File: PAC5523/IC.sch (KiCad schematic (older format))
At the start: 17 parts

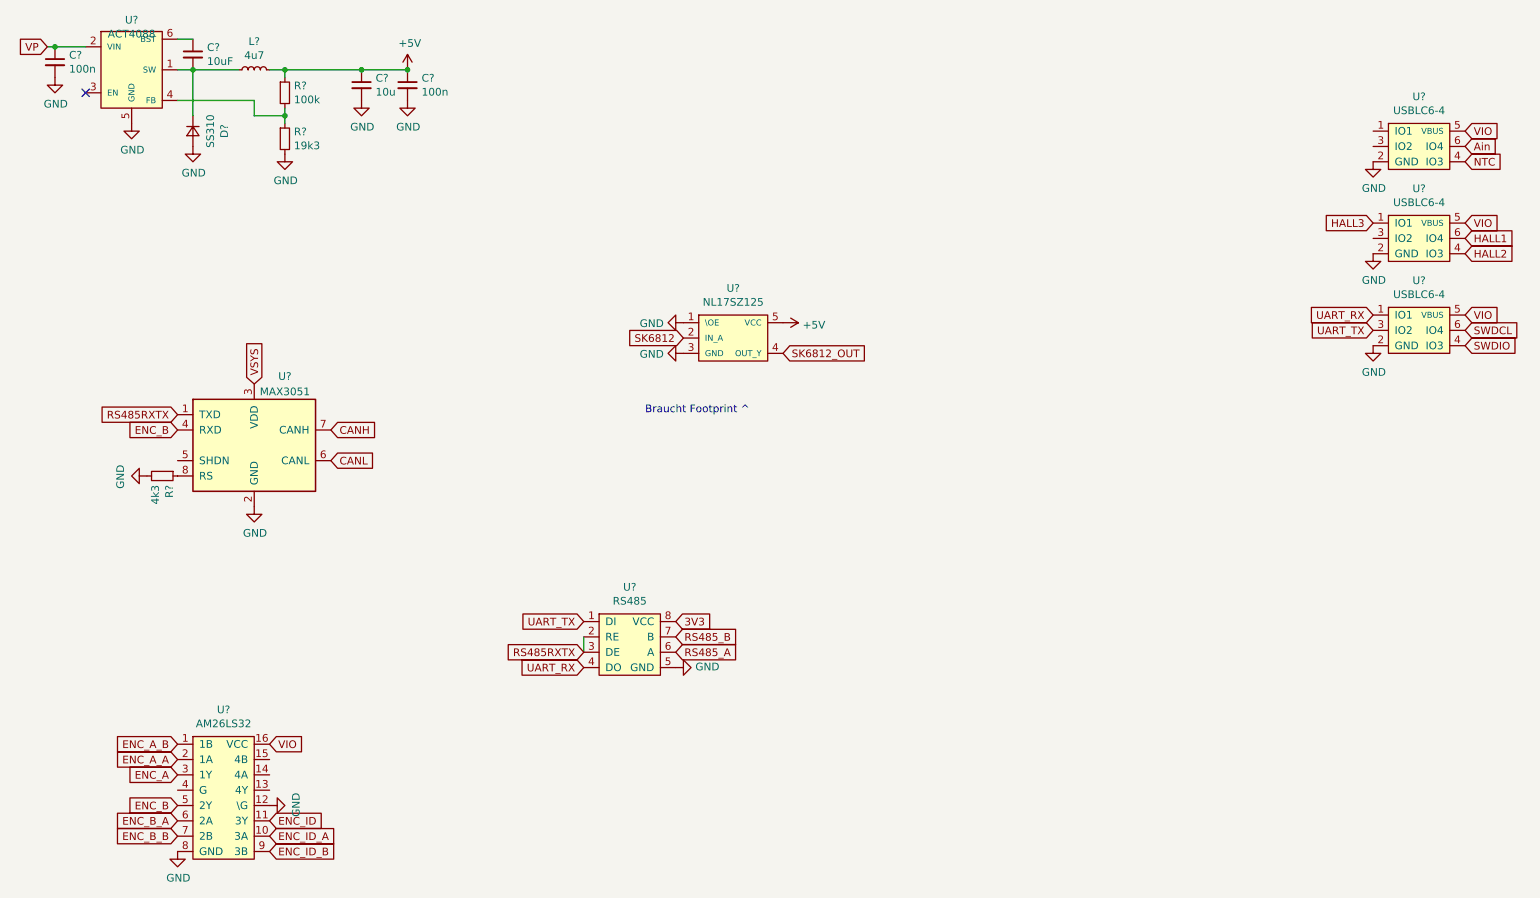
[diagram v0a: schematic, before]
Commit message: updated schematic
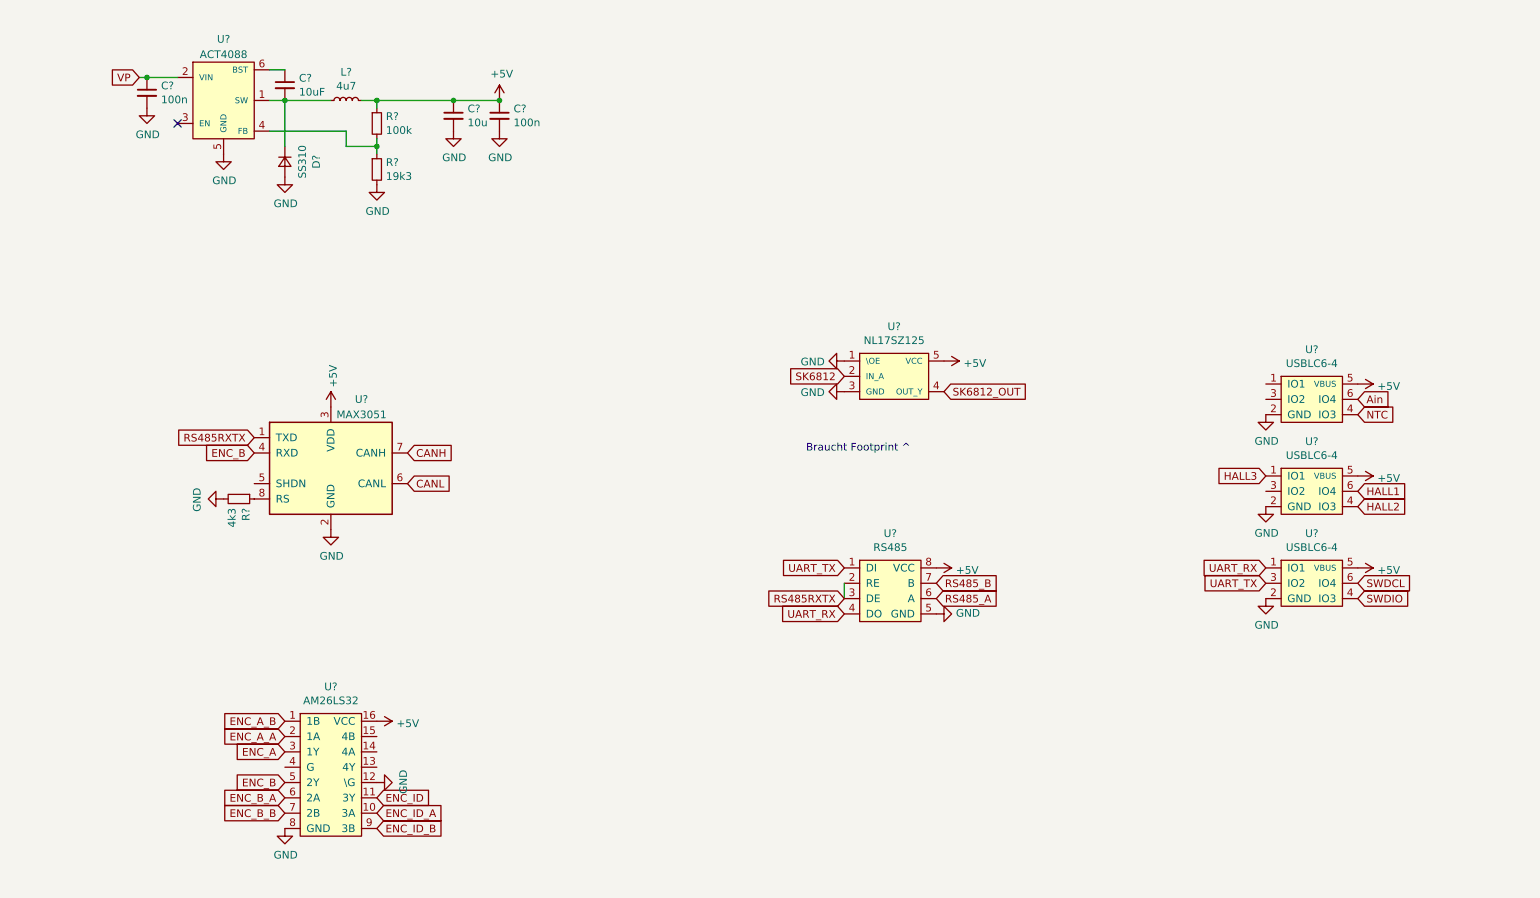
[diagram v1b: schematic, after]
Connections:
- net 3V3 is gone; now on net +5V: U?.8 (VCC)
- net VIO is gone; now on net +5V: U?.16 (VCC), U?.5 (VBUS), U?.5 (VBUS), U?.5 (VBUS)
- net VSYS is gone; now on net +5V: U?.3 (VDD)
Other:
- moved on the sheet: C?, D?, L?, R?, U?

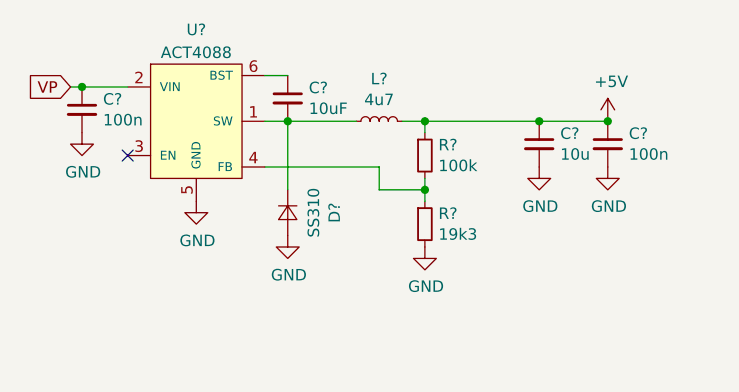
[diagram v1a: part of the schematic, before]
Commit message: updated schematic
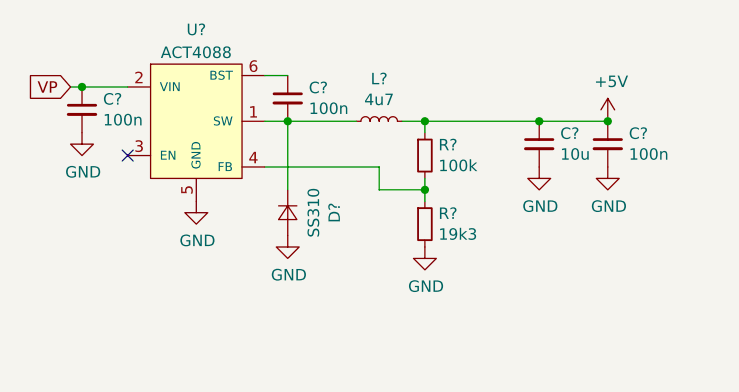
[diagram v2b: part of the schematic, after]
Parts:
- C?: value 10uF -> 100n; footprint Capacitor_SMD:C_0805_2012Metric -> Capacitor_SMD:C_0603_1608Metric
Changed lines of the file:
@@
 P 2550 1300
 F 0 "C?" H 2642 1346 50  0000 L CNN
-F 1 "10uF" H 2642 1255 50  0000 L CNN
-F 2 "Capacitor_SMD:C_0805_2012Metric" H 2550 1300 50  0001 C CNN
+F 1 "100n" H 2642 1255 50  0000 L CNN
+F 2 "Capacitor_SMD:C_0603_1608Metric" H 2550 1300 50  0001 C CNN
 F 3 "~" H 2550 1300 50  0001 C CNN
 	1    2550 1300
